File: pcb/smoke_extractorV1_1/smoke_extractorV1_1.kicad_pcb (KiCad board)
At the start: 2 copper layers, 47 x 35 mm, 48 parts, among them J1 USB_C_Receptacle, J2 Screw_Terminal_01x02, Q1 AO3400A, U1 LMV331, U2 RA11131100, U3 MP1542, U4 LMV331, U5 LMV331, U6 STBP120

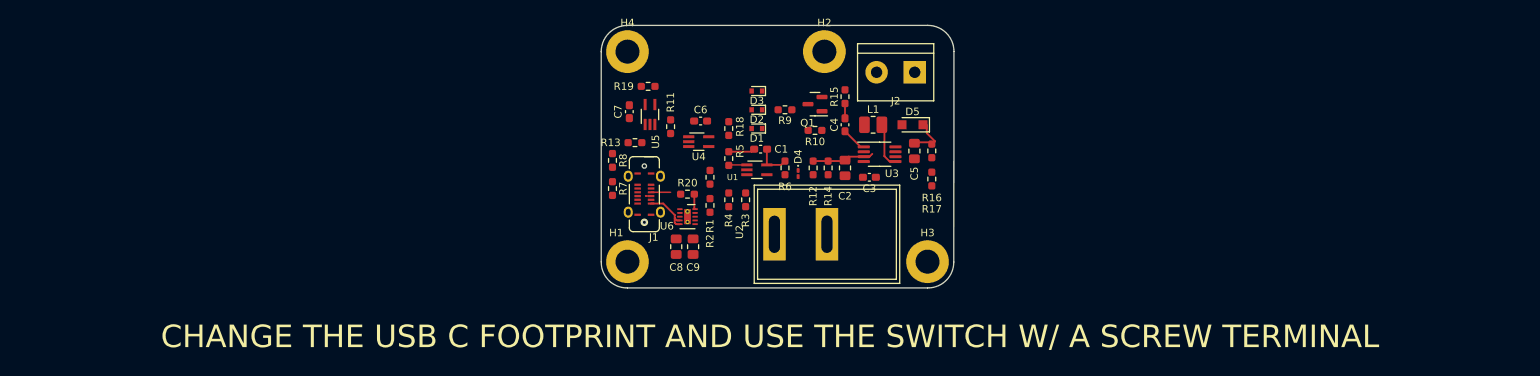
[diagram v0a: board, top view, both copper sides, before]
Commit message: More improvements in the pcb design
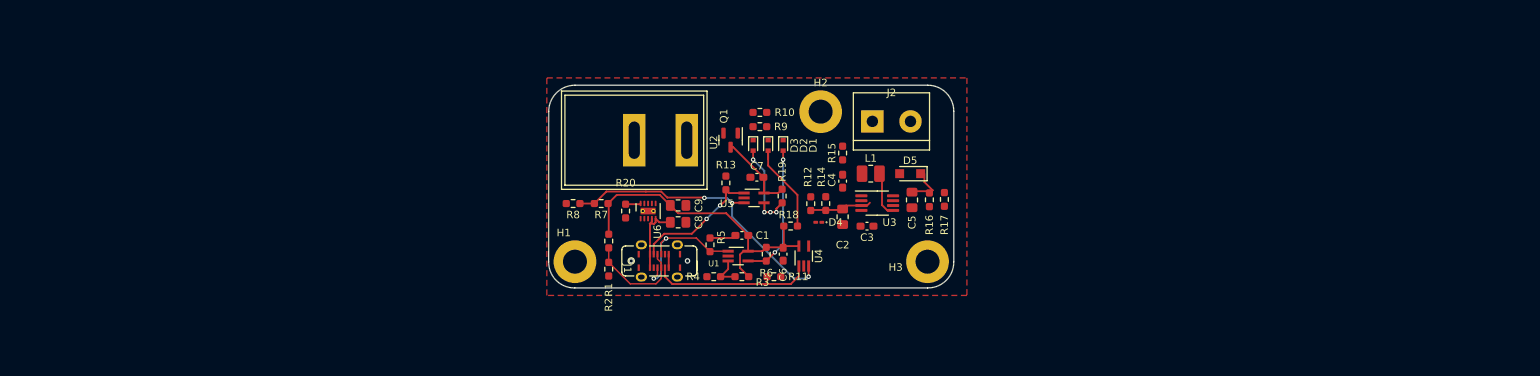
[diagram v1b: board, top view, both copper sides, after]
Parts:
- removed H4: MountingHole_Pad, MountingHole:MountingHole_3.2mm_M3_ISO7380_Pad
- moved R11 24.3 mm to (122.3, 121.5), turned to 180 degrees
- moved R19 23.1 mm to (123.4, 110.8), turned to 90 degrees
- moved C6 20.9 mm to (123.5, 118.5), turned to -90 degrees
- moved U4 20.7 mm to (126.2, 118.8), turned to 90 degrees
- moved C7 19.1 mm to (120.0, 108.2), turned to 180 degrees
- moved U5 17.8 mm to (119.6, 111.0), turned to 0 degrees
- moved R1 16.0 mm to (100.2, 116.8)
- moved R2 16.0 mm to (100.2, 120.5)
- moved R18 15.4 mm to (124.5, 114.8), turned to 180 degrees
- moved R13 13.3 mm to (115.9, 109.0), turned to -90 degrees
- moved Q1 12.2 mm to (116.5, 103.3), turned to -90 degrees
- moved C1 11.8 mm to (118.0, 116.0)
- moved R5 11.8 mm to (113.8, 117.2)
- moved R6 11.8 mm to (121.2, 118.5)
- moved U1 11.8 mm to (117.5, 118.8)
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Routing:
- net VBUS_RAW: track 4.79 -> 53.2 mm
- net V_CC_REF: track 0.00 -> 39.6 mm, vias 0 -> 3
- net CC1: track 0.00 -> 22.2 mm
- net CHG_DET: track 0.00 -> 18.1 mm, vias 0 -> 2
- net CC2: track 0.00 -> 17.5 mm, vias 0 -> 2
- net D-: track 3.20 -> 19.4 mm, vias 0 -> 2
- net CC2_DET: track 0.00 -> 13.2 mm, vias 0 -> 4
- net CC1_DET: track 0.00 -> 12.8 mm
- net D+: track 2.60 -> 13.9 mm
- net Net-(C8-Pad1): track 6.38 -> 12.0 mm
- net VDAT_REF: track 0.00 -> 4.44 mm
- net Net-(C4-Pad1): track 3.36 -> 0.41 mm
- net Net-(C4-Pad2): track 1.98 -> 0.00 mm
- added copper zone on F.Cu, net GND
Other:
- board size 47 x 35 mm -> 54 x 27 mm
- board text removed: "CHANGE THE USB C FOOTPRINT AND USE THE SWITCH W/ A SCREW TERMINAL"
